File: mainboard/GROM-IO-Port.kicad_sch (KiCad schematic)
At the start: 27 parts, among them J13 I/O Port, J15 GROM Port, U14 74LS00, U15 74LS04, U18 74LS00, U22 74LS04, U3 74LS04, U4 74LS32, U41 74LS244, U42 74LS367, U43 74LS367

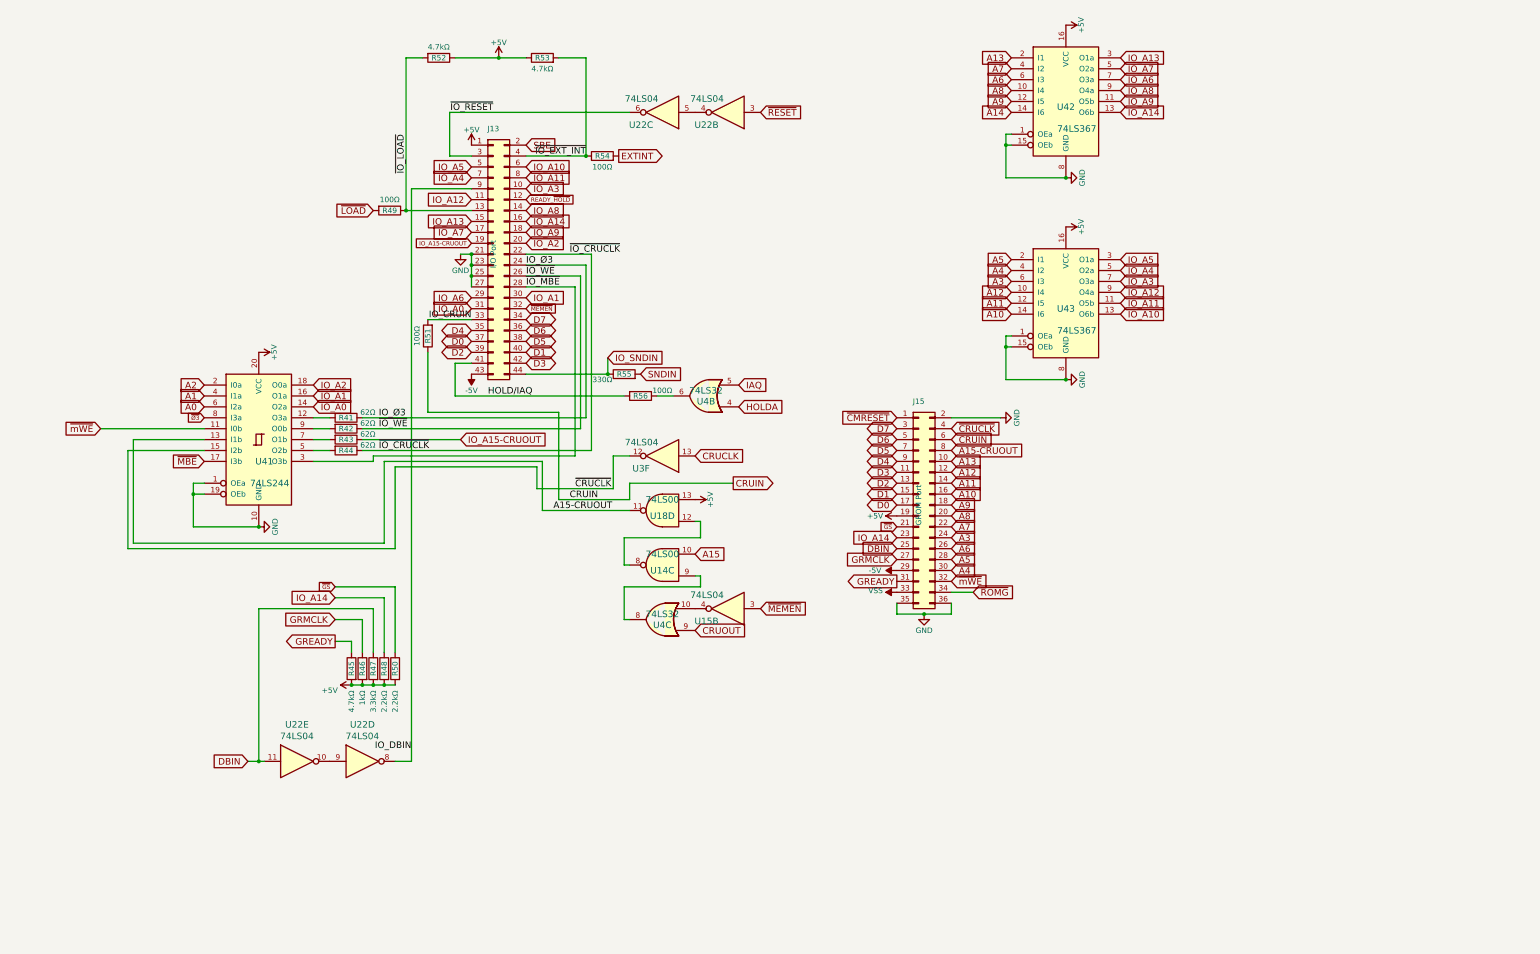
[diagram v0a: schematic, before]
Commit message: layout work
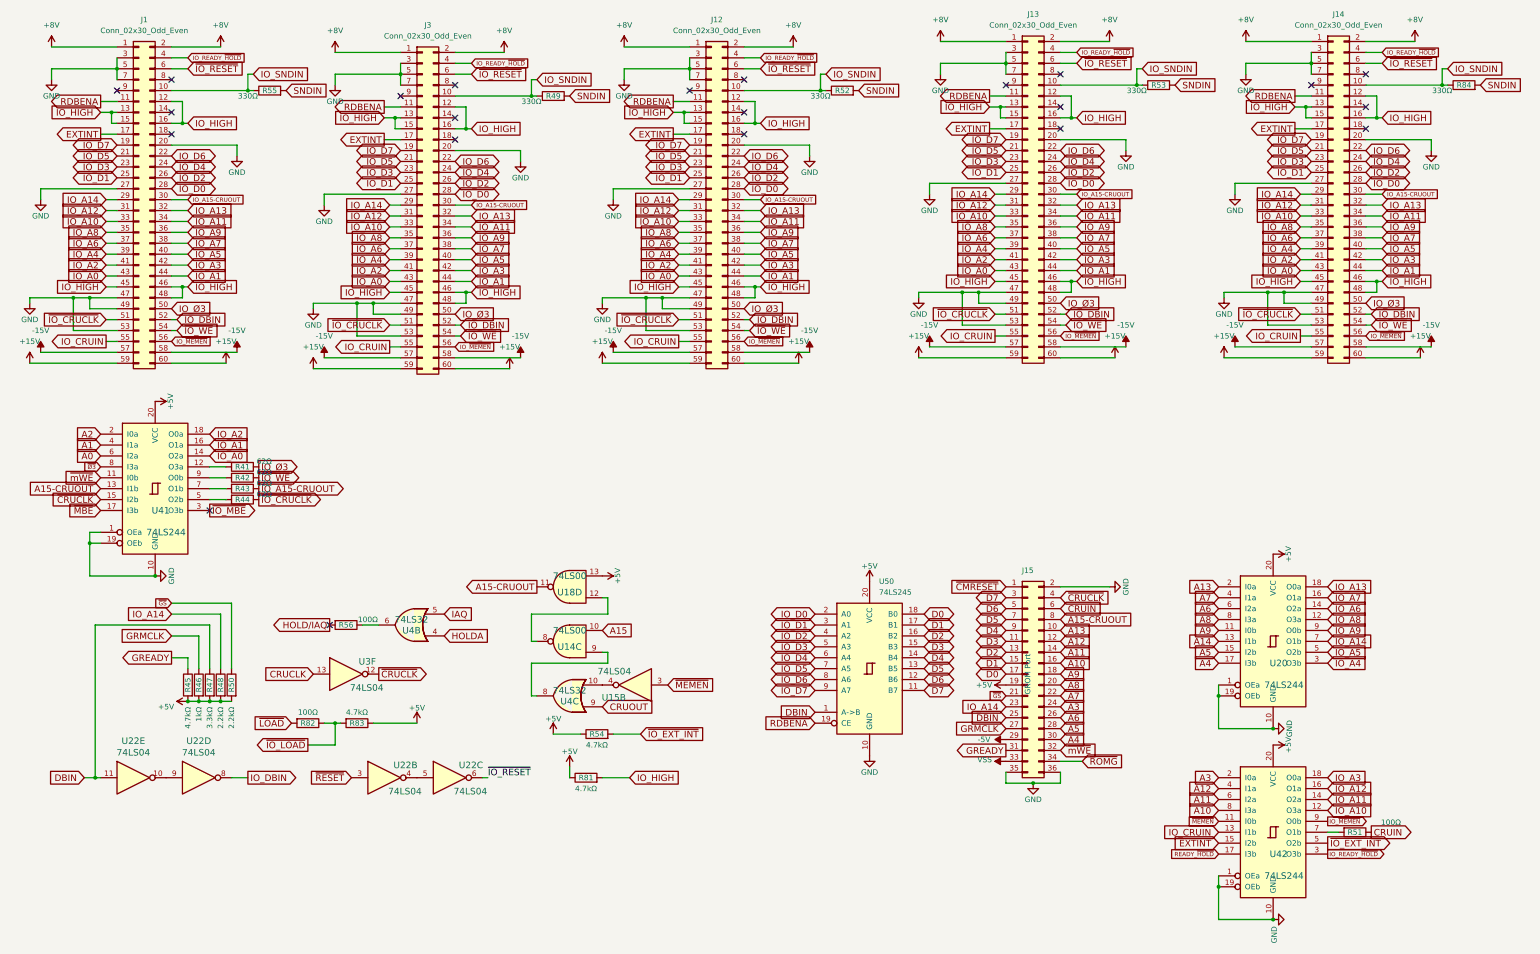
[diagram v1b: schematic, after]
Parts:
- removed J13: I/O Port, Custom:STD_DDW_CARDEDGE_44, symbol Connector_Generic:Conn_02x22_Odd_Even
- removed U42, U43: 74LS367, Custom:STD_DDW_DIP16, symbol 74xx:74LS367
- added J1, J12, J13, J14, J3: Conn_02x30_Odd_Even, Custom:STD_DDW_CARDEDGE60, symbol Connector_Generic:Conn_02x30_Odd_Even
- added R81, R83: 4.7kΩ, Custom:STD_DDW_RESISTOR, symbol Device:R
- added R82: 100Ω, Custom:STD_DDW_RESISTOR, symbol Device:R
- added R84: 330Ω, Custom:STD_DDW_RESISTOR, symbol Device:R
- added U20, U42: 74LS244, Custom:STD_DDW_DIP20, symbol 74xx:74LS244
- added U50: 74LS245, Custom:STD_DDW_DIP20, symbol 74xx:74LS245
- R49: value 100Ω -> 330Ω
- R52, R53: value 4.7kΩ -> 330Ω
- R54: value 100Ω -> 4.7kΩ
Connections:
- net +5V: now also R54.1, R81.1, R83.1, U20.20 (VCC), U42.20 (VCC), U50.20 (VCC); no longer R52.1, R53.1
- net A10: now also U42.8 (I3a)
- net A11: now also U42.6 (I2a)
- net A12: now also U42.4 (I1a)
- net A13: now also U20.2 (I0a)
- net A14: now also U20.13 (I1b)
- net A3: now also U42.2 (I0a)
- net A4: now also U20.17 (I3b)
- net A5: now also U20.15 (I2b)
- net A6: now also U20.6 (I2a)
- net A7: now also U20.4 (I1a)
- net A8: now also U20.8 (I3a)
- net A9: now also U20.11 (I0b)
- net D0: now also U50.18 (B0)
- net D1: now also U50.17 (B1)
- net D2: now also U50.16 (B2)
- net D3: now also U50.15 (B3)
- net D4: now also U50.14 (B4)
- net D5: now also U50.13 (B5)
- net D6: now also U50.12 (B6)
- net D7: now also U50.11 (B7)
- net DBIN: now also U50.1 (A->B)
- net EXTINT: now also J1.17 (Pin_17), J12.17 (Pin_17), J13.17 (Pin_17), J14.17 (Pin_17), J3.17 (Pin_17), U42.15 (I2b); no longer R54.2
- net GND: now also J1.20 (Pin_20), J1.27 (Pin_27), J1.3 (Pin_3), J1.47 (Pin_47), J1.49 (Pin_49), J1.5 (Pin_5), J1.53 (Pin_53), J1.7 (Pin_7), J12.20 (Pin_20), J12.27 (Pin_27), J12.3 (Pin_3), J12.47 (Pin_47), J12.49 (Pin_49), J12.5 (Pin_5), J12.53 (Pin_53), J12.7 (Pin_7), J13.20 (Pin_20), J13.27 (Pin_27), J13.3 (Pin_3), J13.47 (Pin_47), J13.49 (Pin_49), J13.5 (Pin_5), J13.53 (Pin_53), J13.7 (Pin_7), J14.20 (Pin_20), J14.27 (Pin_27), J14.3 (Pin_3), J14.47 (Pin_47), J14.49 (Pin_49), J14.5 (Pin_5), J14.53 (Pin_53), J14.7 (Pin_7), J3.20 (Pin_20), J3.27 (Pin_27), J3.3 (Pin_3), J3.47 (Pin_47), J3.49 (Pin_49), J3.5 (Pin_5), J3.53 (Pin_53), J3.7 (Pin_7), U20.1 (OEa), U20.10 (GND), U20.19 (OEb), U42.1 (OEa), U42.10 (GND), U42.19 (OEb), U50.10 (GND)
- net IO_A0: now also J1.43 (Pin_43), J12.43 (Pin_43), J13.43 (Pin_43), J14.43 (Pin_43), J3.43 (Pin_43)
- net IO_A1: now also J1.44 (Pin_44), J12.44 (Pin_44), J13.44 (Pin_44), J14.44 (Pin_44), J3.44 (Pin_44)
- net IO_A10: now also J1.33 (Pin_33), J12.33 (Pin_33), J13.33 (Pin_33), J14.33 (Pin_33), J3.33 (Pin_33), U42.12 (O3a)
- net IO_A11: now also J1.34 (Pin_34), J12.34 (Pin_34), J13.34 (Pin_34), J14.34 (Pin_34), J3.34 (Pin_34), U42.14 (O2a)
- net IO_A12: now also J1.31 (Pin_31), J12.31 (Pin_31), J13.31 (Pin_31), J14.31 (Pin_31), J3.31 (Pin_31), U42.16 (O1a)
- net IO_A13: now also J1.32 (Pin_32), J12.32 (Pin_32), J13.32 (Pin_32), J14.32 (Pin_32), J3.32 (Pin_32), U20.18 (O0a)
- net IO_A14: now also J1.29 (Pin_29), J12.29 (Pin_29), J13.29 (Pin_29), J14.29 (Pin_29), J3.29 (Pin_29), U20.7 (O1b)
- net IO_A15-CRUOUT: now also J1.30 (Pin_30), J12.30 (Pin_30), J13.30 (Pin_30), J14.30 (Pin_30), J3.30 (Pin_30)
- net IO_A2: now also J1.41 (Pin_41), J12.41 (Pin_41), J13.41 (Pin_41), J14.41 (Pin_41), J3.41 (Pin_41)
- net IO_A3: now also J1.42 (Pin_42), J12.42 (Pin_42), J13.42 (Pin_42), J14.42 (Pin_42), J3.42 (Pin_42), U42.18 (O0a)
- net IO_A4: now also J1.39 (Pin_39), J12.39 (Pin_39), J13.39 (Pin_39), J14.39 (Pin_39), J3.39 (Pin_39), U20.3 (O3b)
- net IO_A5: now also J1.40 (Pin_40), J12.40 (Pin_40), J13.40 (Pin_40), J14.40 (Pin_40), J3.40 (Pin_40), U20.5 (O2b)
- net IO_A6: now also J1.37 (Pin_37), J12.37 (Pin_37), J13.37 (Pin_37), J14.37 (Pin_37), J3.37 (Pin_37), U20.14 (O2a)
- net IO_A7: now also J1.38 (Pin_38), J12.38 (Pin_38), J13.38 (Pin_38), J14.38 (Pin_38), J3.38 (Pin_38), U20.16 (O1a)
- net IO_A8: now also J1.35 (Pin_35), J12.35 (Pin_35), J13.35 (Pin_35), J14.35 (Pin_35), J3.35 (Pin_35), U20.12 (O3a)
- net IO_A9: now also J1.36 (Pin_36), J12.36 (Pin_36), J13.36 (Pin_36), J14.36 (Pin_36), J3.36 (Pin_36), U20.9 (O0b)
- net IO_CRUIN: now also J1.55 (Pin_55), J12.55 (Pin_55), J13.55 (Pin_55), J14.55 (Pin_55), J3.55 (Pin_55), U42.13 (I1b); no longer R51.2
- net IO_DBIN: now also J1.52 (Pin_52), J12.52 (Pin_52), J13.52 (Pin_52), J14.52 (Pin_52), J3.52 (Pin_52)
- net IO_SNDIN: now also R49.1, R52.1, R53.1, J1.10 (Pin_10), J12.10 (Pin_10), J13.10 (Pin_10), J14.10 (Pin_10), J3.10 (Pin_10), R84.1
- net IO_Ø3: now also J1.50 (Pin_50), J12.50 (Pin_50), J13.50 (Pin_50), J14.50 (Pin_50), J3.50 (Pin_50)
- net READY_~{HOLD}: now also U42.17 (I3b)
- net SNDIN: now also R49.2, R52.2, R53.2, R84.2
- net ~{IO_CRUCLK}: now also J1.51 (Pin_51), J12.51 (Pin_51), J13.51 (Pin_51), J14.51 (Pin_51), J3.51 (Pin_51)
- net ~{IO_EXT_INT}: now also R54.2, U42.5 (O2b); no longer R53.2, R54.1
- net ~{IO_LOAD}: now also R82.1, R83.2; no longer R49.1, R52.2
- net ~{IO_RESET}: now also J1.6 (Pin_6), J12.6 (Pin_6), J13.6 (Pin_6), J14.6 (Pin_6), J3.6 (Pin_6)
- net ~{IO_WE}: now also J1.54 (Pin_54), J12.54 (Pin_54), J13.54 (Pin_54), J14.54 (Pin_54), J3.54 (Pin_54)
- net ~{LOAD}: now also R82.2; no longer R49.2
- net ~{MEMEN}: now also U42.11 (I0b)
- net HOLD/IAQ renamed HOLD/IAQ
- new net: R51.2, U42.7 (O1b)
- new net +15V: J1.59 (Pin_59), J1.60 (Pin_60), J12.59 (Pin_59), J12.60 (Pin_60), J13.59 (Pin_59), J13.60 (Pin_60), J14.59 (Pin_59), J14.60 (Pin_60), J3.59 (Pin_59), J3.60 (Pin_60)
- new net +8V: J1.1 (Pin_1), J1.2 (Pin_2), J12.1 (Pin_1), J12.2 (Pin_2), J13.1 (Pin_1), J13.2 (Pin_2), J14.1 (Pin_1), J14.2 (Pin_2), J3.1 (Pin_1), J3.2 (Pin_2)
- new net -15V: J1.57 (Pin_57), J1.58 (Pin_58), J12.57 (Pin_57), J12.58 (Pin_58), J13.57 (Pin_57), J13.58 (Pin_58), J14.57 (Pin_57), J14.58 (Pin_58), J3.57 (Pin_57), J3.58 (Pin_58)
- new net IO_D0: J1.28 (Pin_28), J12.28 (Pin_28), J13.28 (Pin_28), J14.28 (Pin_28), J3.28 (Pin_28), U50.2 (A0)
- new net IO_D1: J1.25 (Pin_25), J12.25 (Pin_25), J13.25 (Pin_25), J14.25 (Pin_25), J3.25 (Pin_25), U50.3 (A1)
- new net IO_D2: J1.26 (Pin_26), J12.26 (Pin_26), J13.26 (Pin_26), J14.26 (Pin_26), J3.26 (Pin_26), U50.4 (A2)
- new net IO_D3: J1.23 (Pin_23), J12.23 (Pin_23), J13.23 (Pin_23), J14.23 (Pin_23), J3.23 (Pin_23), U50.5 (A3)
- new net IO_D4: J1.24 (Pin_24), J12.24 (Pin_24), J13.24 (Pin_24), J14.24 (Pin_24), J3.24 (Pin_24), U50.6 (A4)
- new net IO_D5: J1.21 (Pin_21), J12.21 (Pin_21), J13.21 (Pin_21), J14.21 (Pin_21), J3.21 (Pin_21), U50.7 (A5)
- new net IO_D6: J1.22 (Pin_22), J12.22 (Pin_22), J13.22 (Pin_22), J14.22 (Pin_22), J3.22 (Pin_22), U50.8 (A6)
- new net IO_D7: J1.19 (Pin_19), J12.19 (Pin_19), J13.19 (Pin_19), J14.19 (Pin_19), J3.19 (Pin_19), U50.9 (A7)
- new net IO_HIGH: J1.12 (Pin_12), J1.13 (Pin_13), J1.15 (Pin_15), J1.16 (Pin_16), J1.45 (Pin_45), J1.46 (Pin_46), J1.48 (Pin_48), J12.12 (Pin_12), J12.13 (Pin_13), J12.15 (Pin_15), J12.16 (Pin_16), J12.45 (Pin_45), J12.46 (Pin_46), J12.48 (Pin_48), J13.12 (Pin_12), J13.13 (Pin_13), J13.15 (Pin_15), J13.16 (Pin_16), J13.45 (Pin_45), J13.46 (Pin_46), J13.48 (Pin_48), J14.12 (Pin_12), J14.13 (Pin_13), J14.15 (Pin_15), J14.16 (Pin_16), J14.45 (Pin_45), J14.46 (Pin_46), J14.48 (Pin_48), J3.12 (Pin_12), J3.13 (Pin_13), J3.15 (Pin_15), J3.16 (Pin_16), J3.45 (Pin_45), J3.46 (Pin_46), J3.48 (Pin_48), R81.2
- new net IO_READY_~{HOLD}: J1.4 (Pin_4), J12.4 (Pin_4), J13.4 (Pin_4), J14.4 (Pin_4), J3.4 (Pin_4), U42.3 (O3b)
- new net IO_~{MEMEN}: J1.56 (Pin_56), J12.56 (Pin_56), J13.56 (Pin_56), J14.56 (Pin_56), J3.56 (Pin_56), U42.9 (O0b)
- new net RDBENA: J1.11 (Pin_11), J12.11 (Pin_11), J13.11 (Pin_11), J14.11 (Pin_11), J3.11 (Pin_11), U50.19 (CE)
- no-connect marks 0 -> 22
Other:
- moved on the sheet: J15, R41, R42, R43, R44, R45, R46, R47, R48, R50, R51, R55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

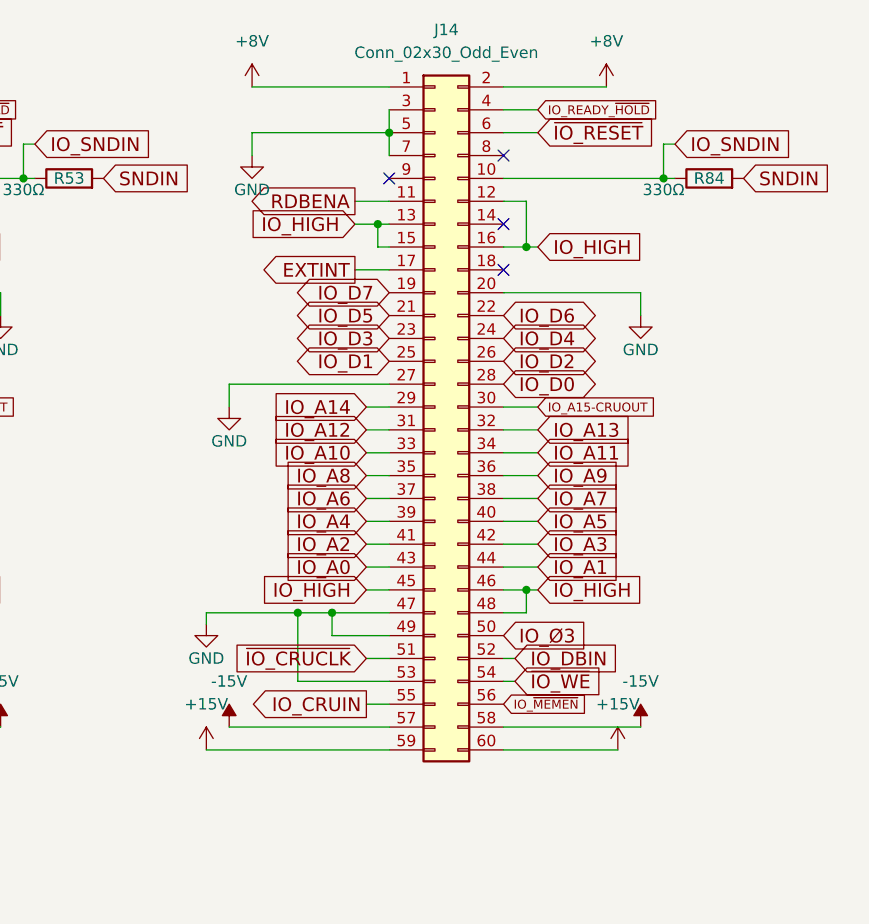
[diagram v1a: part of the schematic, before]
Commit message: layout work
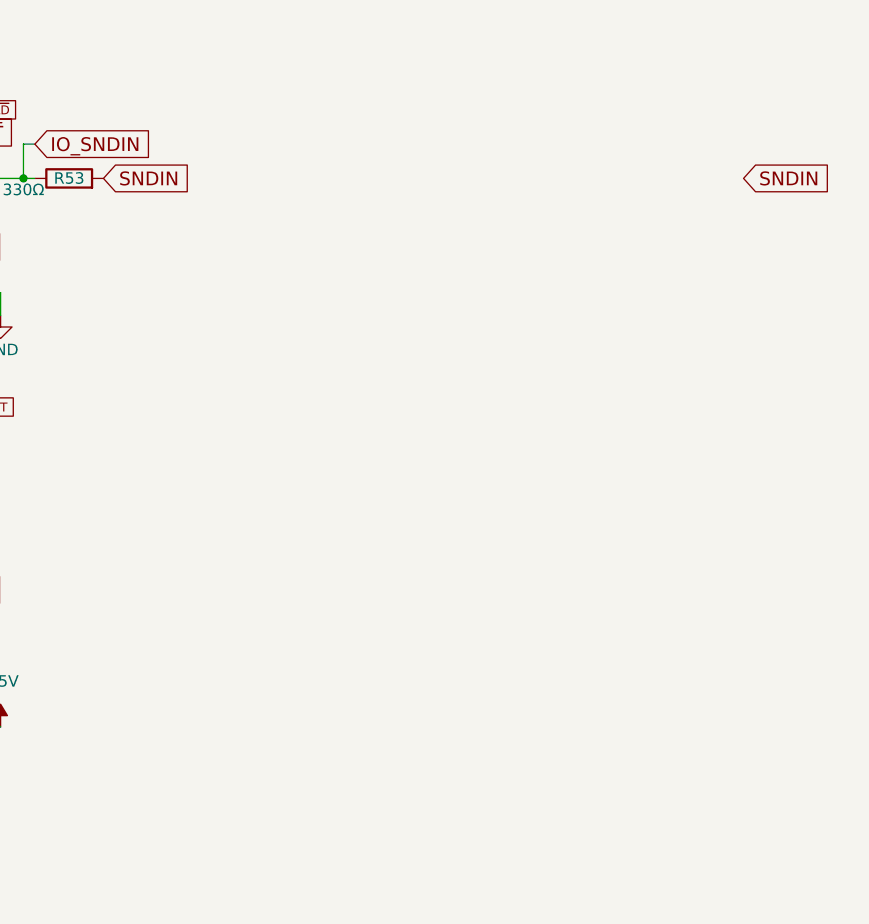
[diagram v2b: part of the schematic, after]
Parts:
- removed J14: Conn_02x30_Odd_Even, Custom:STD_DDW_CARDEDGE60, symbol Connector_Generic:Conn_02x30_Odd_Even
- removed R84: 330Ω, Custom:STD_DDW_RESISTOR, symbol Device:R
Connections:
- no-connect marks 22 -> 18
